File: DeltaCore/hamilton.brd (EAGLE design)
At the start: 45 x 41.5 mm, 70 parts, among them Q3 MOSFET-NCHANNEL_SOT23-3, Q4 MOSFET-NCHANNEL_SOT23-3, Q5 MOSFET-NCHANNEL_SOT23-3, Q6 MOSFET-NCHANNEL_SOT23-3, Q7 NFET_AON7408, Q8 NFET_AON7408, U1 SAMR21, U10 PCA9557, U3 MMA7660FC, U4 AT30TS74, U5 MCP73871-2AAI/ML, U7 BQ29718, U8 MCP1824ST-3302E/DB, U9 TPS61090, X1 XTAL

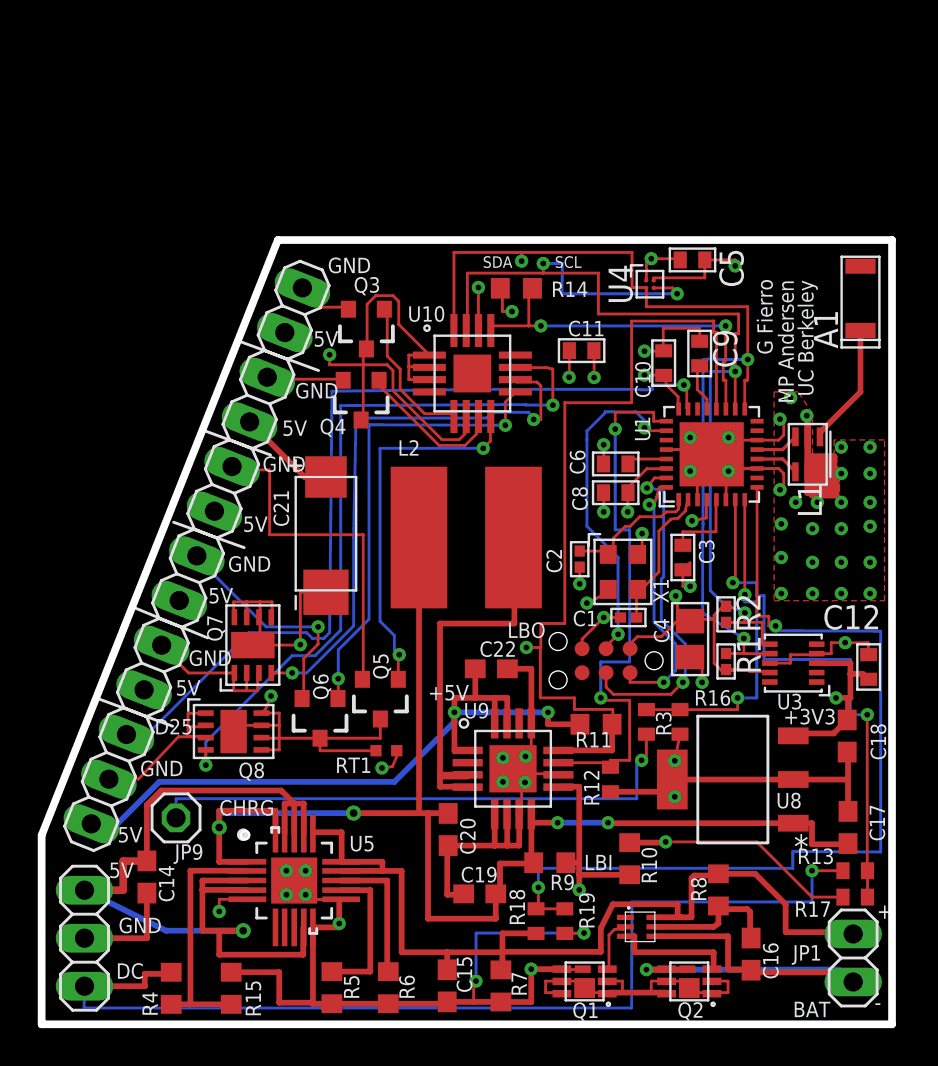
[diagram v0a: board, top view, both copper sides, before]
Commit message: next version
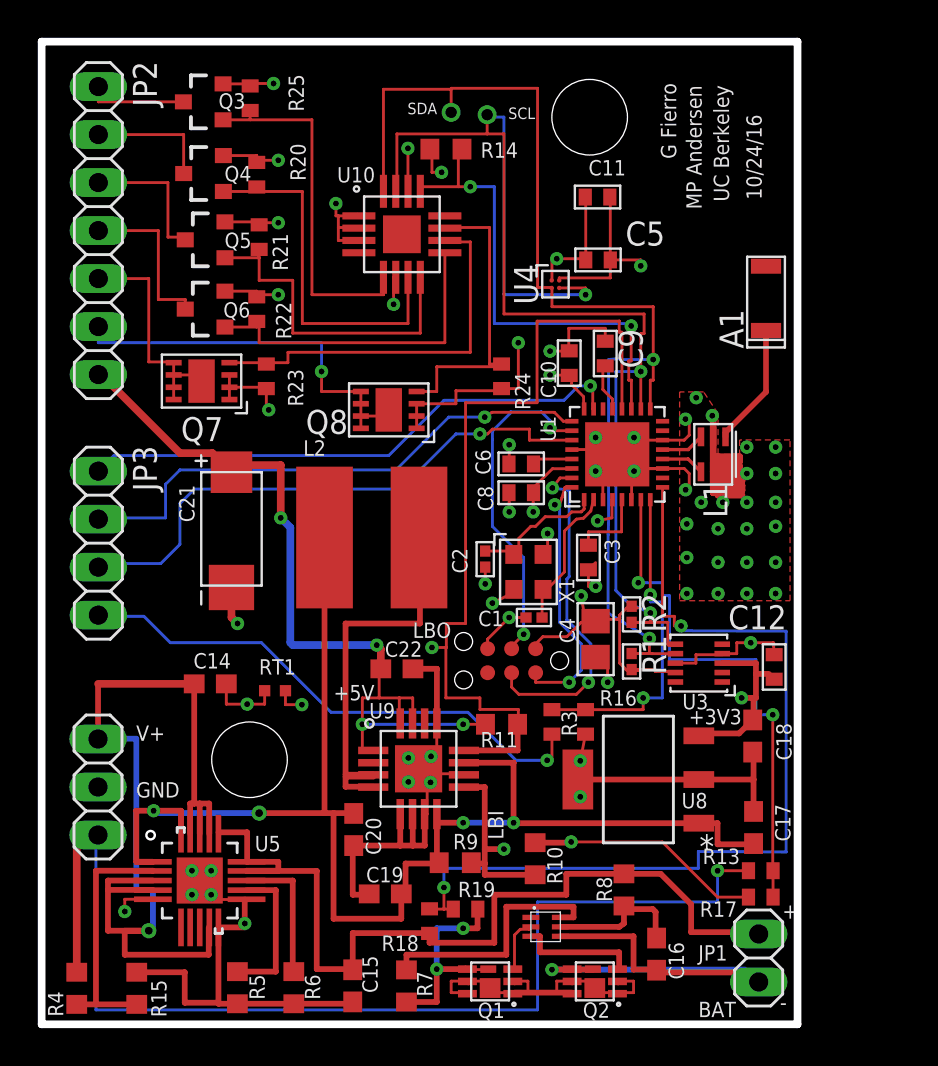
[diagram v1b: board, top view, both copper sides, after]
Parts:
- removed JP4: insole3, pinhead:1X02
- removed JP5: insole4, pinhead:1X02
- removed JP6: insole/wrist, pinhead:1X02
- removed JP7: insole/fan/pwm, pinhead:1X03
- removed JP9: (no value), pinhead:1X01
- removed R12: 10k, resistor:R0402
- added R20, R21, R22, R23, R24, R25: 10k, resistor:R0402
- JP2: value insole1 -> (none); device pinhead:1X02 -> pinhead:1X07
- JP3: value insole2 -> (none); device pinhead:1X02 -> pinhead:1X04
- moved Q5 26.0 mm to (8.70, 41.5), turned to 90 degrees
- moved Q6 22.4 mm to (8.70, 37.8), turned to 90 degrees
- moved Q8 18.9 mm to (18.4, 32.5), turned to 90 degrees
- moved Q3 14.7 mm to (8.60, 48.8), turned to 90 degrees
- moved Q4 14.5 mm to (8.62, 45.0), turned to 90 degrees
- moved Q7 14.2 mm to (8.46, 34.0), turned to 90 degrees
- moved JP3 11.4 mm to (3.00, 25.5), turned to 270 degrees
- moved JP2 11.2 mm to (3.00, 42.0), turned to 270 degrees
- moved C14 10.8 mm to (8.92, 18.0), turned to 0 degrees
- moved R14 8.26 mm to (21.4, 46.3)
- moved U10 8.26 mm to (19.1, 41.8)
- moved C11 8.17 mm to (29.4, 43.8)
- moved JP8 8.03 mm to (2.98, 12.6)
- moved RT1 6.69 mm to (12.4, 17.7)
- moved R18 5.63 mm to (20.5, 5.46)
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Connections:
- removed net EN: R12.2, U1.25, U9.EN
- removed net N$39: JP7.2, Q8.1, Q8.2, Q8.3
- removed net N$8: JP9.1, R3.2
- new net ADC7: JP3.4, R3.2
- new net D27: JP3.2, U1.25
- new net D28: JP3.3, U1.27
- new net N$11: JP2.5, Q7.5, Q7.6, Q7.7, Q7.8, Q7.PAD
- new net N$26: JP2.6, Q8.5, Q8.6, Q8.7, Q8.8, Q8.PAD
- net 5V: now also JP2.7; no longer JP2.1, JP3.1, JP4.1, JP5.1, JP6.1, JP7.1
- net D25: now also JP3.1; no longer JP7.3
- net GND: now also Q3.2, Q4.2, Q5.2, Q6.2, Q7.1, Q7.2, Q7.3, Q8.1, Q8.2, Q8.3, R20.1, R21.1, R22.1, R23.1, R24.1, R25.1; no longer Q3.3, Q4.3, Q5.3, Q6.3, Q7.5, Q7.6, Q7.7, Q7.8, Q7.PAD, Q8.5, Q8.6, Q8.7, Q8.8, Q8.PAD, R12.1
- net N$14: now also JP2.1, Q3.3; no longer JP2.2, Q3.2
- net N$20: no longer C15.1, JP1.1, R18.1, R8.2, U5.14, U5.15, U5.16
- net N$30: now also R25.2
- net N$31: now also R20.2
- net N$32: now also R21.2
- net N$33: now also R22.2
- net N$34: now also JP2.2, Q4.3; no longer JP3.2, Q4.2
- net N$35: now also JP2.3, Q5.3; no longer JP4.2, Q5.2
- net N$36: now also JP2.4, Q6.3; no longer JP5.2, Q6.2
- net N$37: now also C15.1, JP1.1, R18.1, R8.2, U5.14, U5.15, U5.16; no longer JP6.2, Q7.1, Q7.2, Q7.3
- net N$40: now also R23.2
- net N$41: now also R24.2
- net OUT: now also U9.EN
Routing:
- net N$37: track 8.72 -> 47.6 mm
- net N$20: track 50.4 -> 13.4 mm
- net D28: track 0.00 -> 29.9 mm, vias 0 -> 1
- net EN: track 29.9 -> 0.00 mm, vias 2 -> 0
- net N$8: track 29.3 -> 0.00 mm, vias 1 -> 0
- net D27: track 0.00 -> 28.6 mm, vias 0 -> 1
- net ADC7: track 0.00 -> 28.6 mm, vias 0 -> 1
- net N$41: track 38.6 -> 16.2 mm, vias 2 -> 0
- net GND: track 248.7 -> 226.6 mm, vias 59 -> 64
- net N$26: track 0.00 -> 21.1 mm, vias 0 -> 1
- net D25: track 46.2 -> 29.3 mm
- net SCL: track 55.7 -> 68.6 mm
- net N$11: track 0.00 -> 12.2 mm
- net N$31: track 8.03 -> 19.4 mm
- net N$30: track 8.14 -> 19.2 mm
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- removed copper zone on layer 15, net 5V
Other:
- board size 45 x 41.5 mm -> 40 x 52 mm
- board text added: "10/24/16"
- board text added: "V+"
- board text removed: "5V"
- board text removed: "CHRG"
- board text removed: "D25"
- board text removed: "DC"
- board text removed: "Q7"
- board text removed: "Q8"

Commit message: update
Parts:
- R15: value ?? -> 523k
- R4: value ?? -> 110k
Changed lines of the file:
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@@
 <attribute name="VALUE" x="5.4494" y="3.5074" size="1.016" layer="27" ratio="10" rot="SR0"/>
 </element>
-<element name="R4" library="resistor" package="R0603" value="??" x="1.858" y="1.905" smashed="yes" rot="R90">
+<element name="R4" library="resistor" package="R0603" value="110k" x="1.858" y="1.905" smashed="yes" rot="R90">
 <attribute name="NAME" x="1.1468" y="0.4064" size="0.8128" layer="25" rot="R90"/>
 <attribute name="VALUE" x="3.763" y="1.27" size="1.27" layer="27" rot="R90"/>
 </element>
-<element name="R15" library="resistor" package="R0603" value="??" x="5.033" y="1.905" smashed="yes" rot="R270">
+<element name="R15" library="resistor" package="R0603" value="523k" x="5.033" y="1.905" smashed="yes" rot="R270">
 <attribute name="NAME" x="6.6078" y="0.381" size="0.8128" layer="25" rot="R90"/>
 <attribute name="VALUE" x="3.128" y="2.54" size="1.27" layer="27" rot="R270"/>
@@
 <vertex x="32.084" y="51.894"/>
 <vertex x="32.338" y="20.828"/>
-<vertex x="44.958" y="20.828"/>
-<vertex x="44.958" y="7.62"/>
+<vertex x="40.132" y="20.828"/>
+<vertex x="40.132" y="7.62"/>
 <vertex x="29.21" y="7.112"/>
 <vertex x="29.21" y="4.064"/>
@@
 <vertex x="32.338" y="51.816"/>
 <vertex x="32.338" y="20.574"/>
-<vertex x="44.958" y="20.828"/>
-<vertex x="45.212" y="7.62"/>
+<vertex x="39.878" y="20.828"/>
+<vertex x="40.132" y="7.62"/>
 <vertex x="29.464" y="7.366"/>
 <vertex x="29.464" y="3.81"/>
